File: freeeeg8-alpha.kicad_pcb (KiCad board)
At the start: 2 copper layers, 26 x 26 mm, 33 parts, among them J1 AIN0, J10 GND, J12 STACK_1, J13 STACK_2, J14 XIAO_1, J15 XIAO_2, J2 AIN1, J3 AIN2, J4 AIN3, J5 AIN4, J6 AIN5, J7 AIN6, J8 AIN7, J9 AINREF, U1 ADC, U2 AVDD, U3 DVDD, X1 XTAL

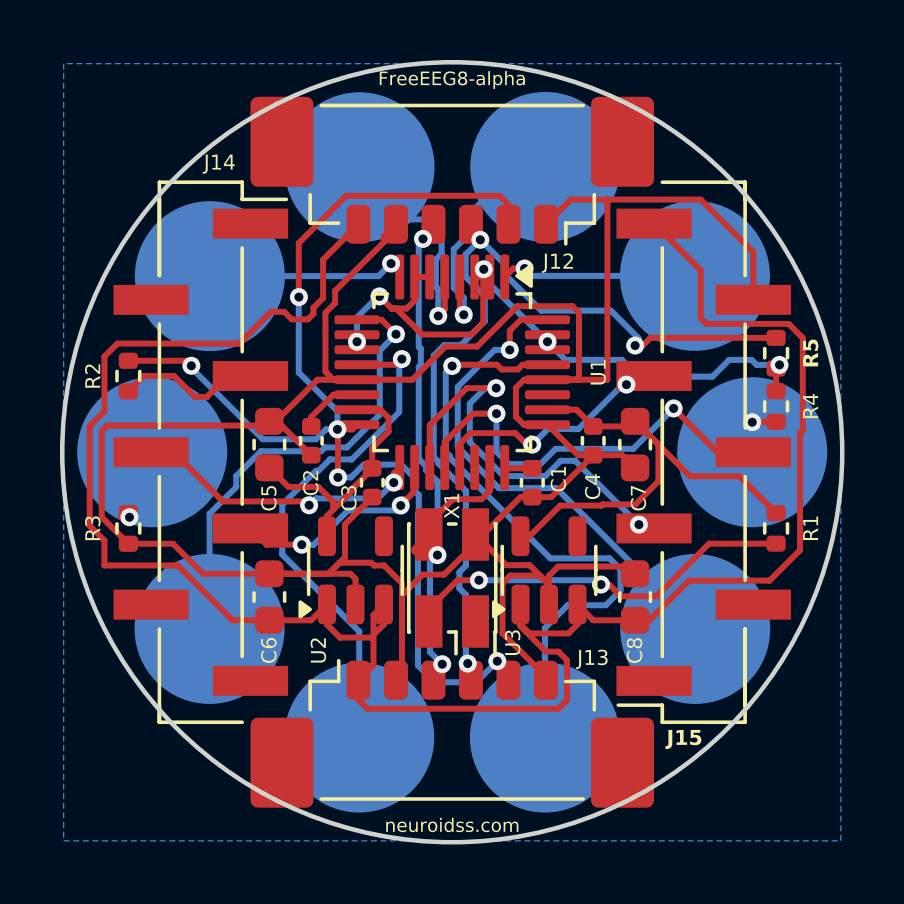
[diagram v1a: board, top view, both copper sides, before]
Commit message: Add files via upload
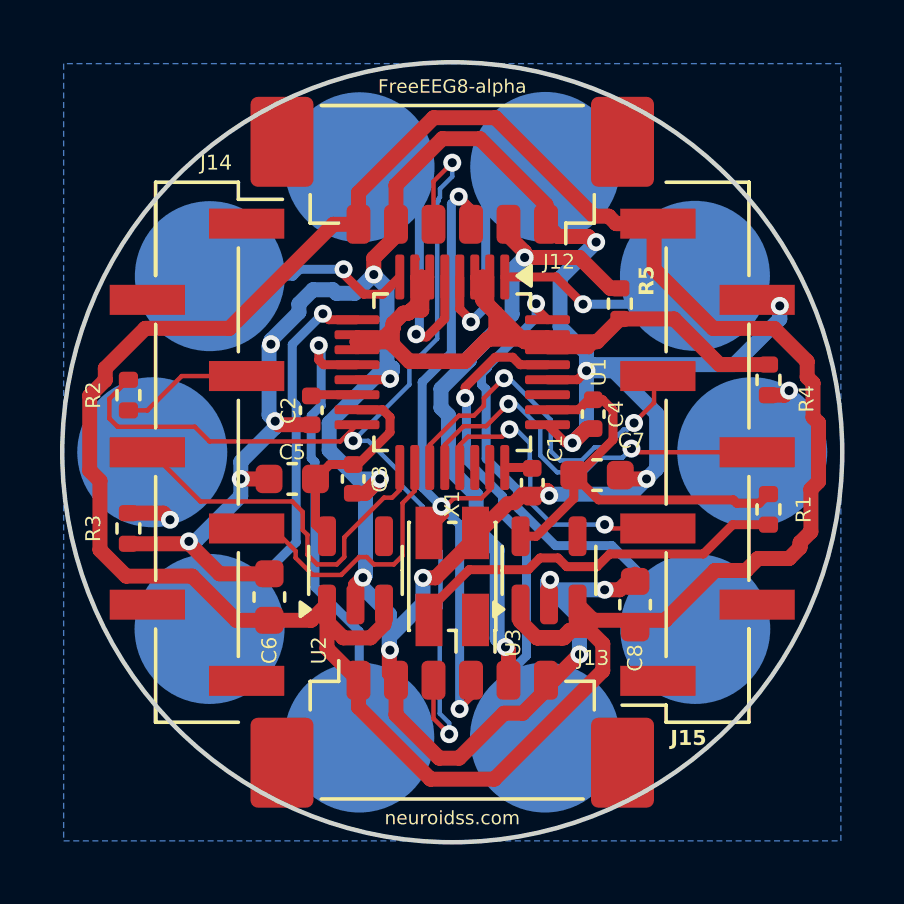
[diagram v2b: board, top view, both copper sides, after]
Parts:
- moved R5 5.46 mm to (5.59, -4.95)
- moved C7 1.63 mm to (4.83, 0.76), turned to 180 degrees
- moved C5 1.37 mm to (-5.33, 0.89), turned to 180 degrees
- moved C2 1.02 mm to (-4.70, -1.40)
- moved R4 0.92 mm to (10.5, -2.41)
- moved C4 0.89 mm to (4.70, -1.27)
- moved R1 0.68 mm to (10.5, 1.91)
- moved C3 0.65 mm to (-3.30, 0.89)
- moved R2 0.64 mm to (-10.8, -1.91)
- moved C8 0.25 mm to (6.10, 5.08)
- moved J14 0.13 mm to (-8.51, 0.00)
- moved J15 0.13 mm to (8.51, 0.00)
- moved X1 0.05 mm to (0.00, 4.14)
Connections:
- J12 pad 2: /SYNC/RESET_ADC -> /AINREF_STACK
- J12 pad 3: /AINREF_STACK -> /XTAL1/CLKIN
- J12 pad 4: /XTAL1/CLKIN -> /SYNC/RESET_ADC
- J13 pad 3: /XTAL1/CLKIN -> /SYNC/RESET_ADC
- J13 pad 4: /AINREF_STACK -> /XTAL1/CLKIN
- J13 pad 5: /SYNC/RESET_ADC -> /AINREF_STACK
- J15 pad 3: /SCLK -> /DIN
- J15 pad 5: /DIN -> /SCLK
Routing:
- net /AINREF: track 25.6 -> 47.6 mm, vias 5 -> 0
- net /5V: track 72.2 -> 87.4 mm
- net /AINREF_STACK: track 29.6 -> 21.3 mm, vias 3 -> 2
- net /GND: track 104.9 -> 112.9 mm, vias 0 -> 19
- net /XTAL1/CLKIN: track 21.5 -> 28.3 mm
- net /AIN0P: track 21.2 -> 16.3 mm
- net /AINREF_POGOPIN: track 1.85 -> 5.05 mm
- net /CS: track 9.72 -> 12.7 mm, vias 2 -> 0
- net /SYNC/RESET_ADC: track 38.9 -> 36.7 mm, vias 5 -> 3
- net /AIN6P: track 15.5 -> 13.4 mm
- net /DRDY: track 7.32 -> 9.42 mm, vias 2 -> 0
- net /AVDD: track 8.82 -> 7.08 mm
- net /AIN7P: track 17.4 -> 15.7 mm
- net /AIN4P: track 7.97 -> 9.58 mm
- net /SCLK: track 14.3 -> 12.7 mm
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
